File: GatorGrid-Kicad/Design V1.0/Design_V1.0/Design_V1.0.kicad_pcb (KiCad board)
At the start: 2 copper layers, 95 x 63 mm, 10 parts, among them J1 Conn_01x02, U1 TP4056

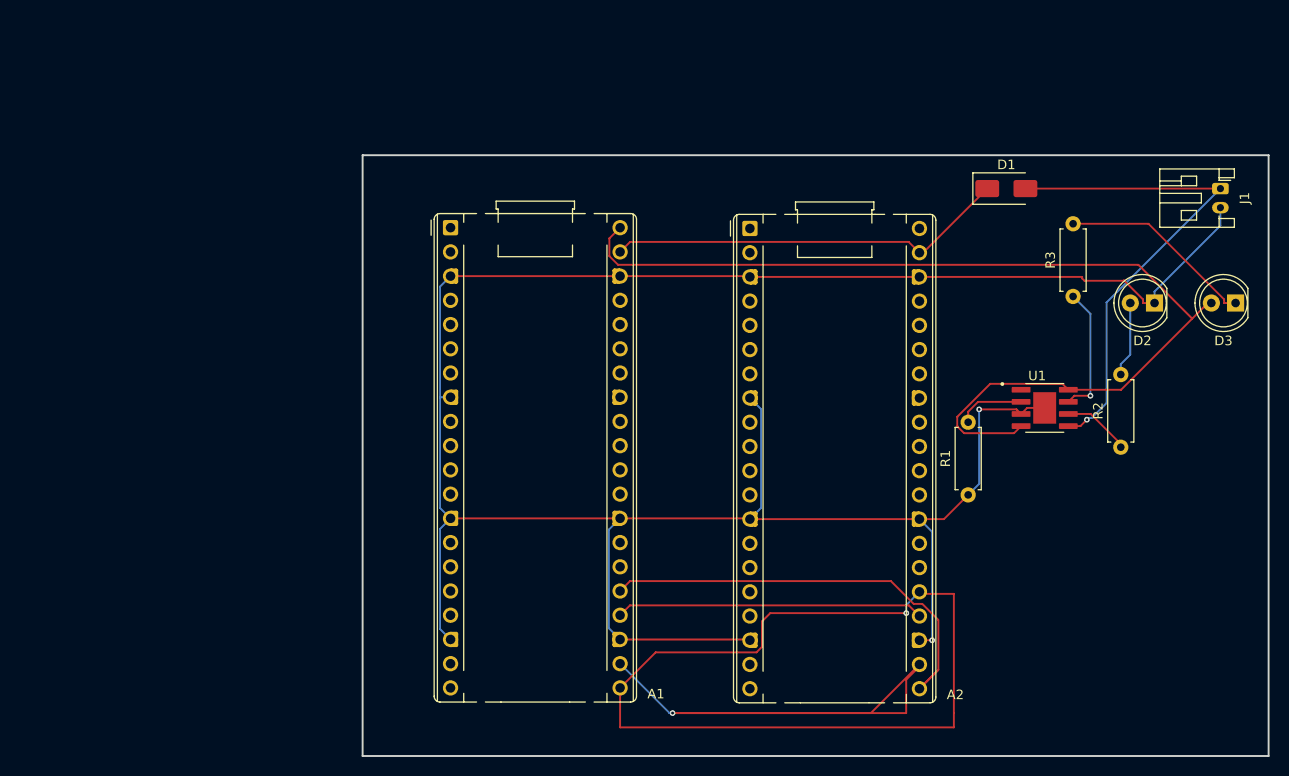
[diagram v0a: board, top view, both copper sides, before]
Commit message: updated PCB
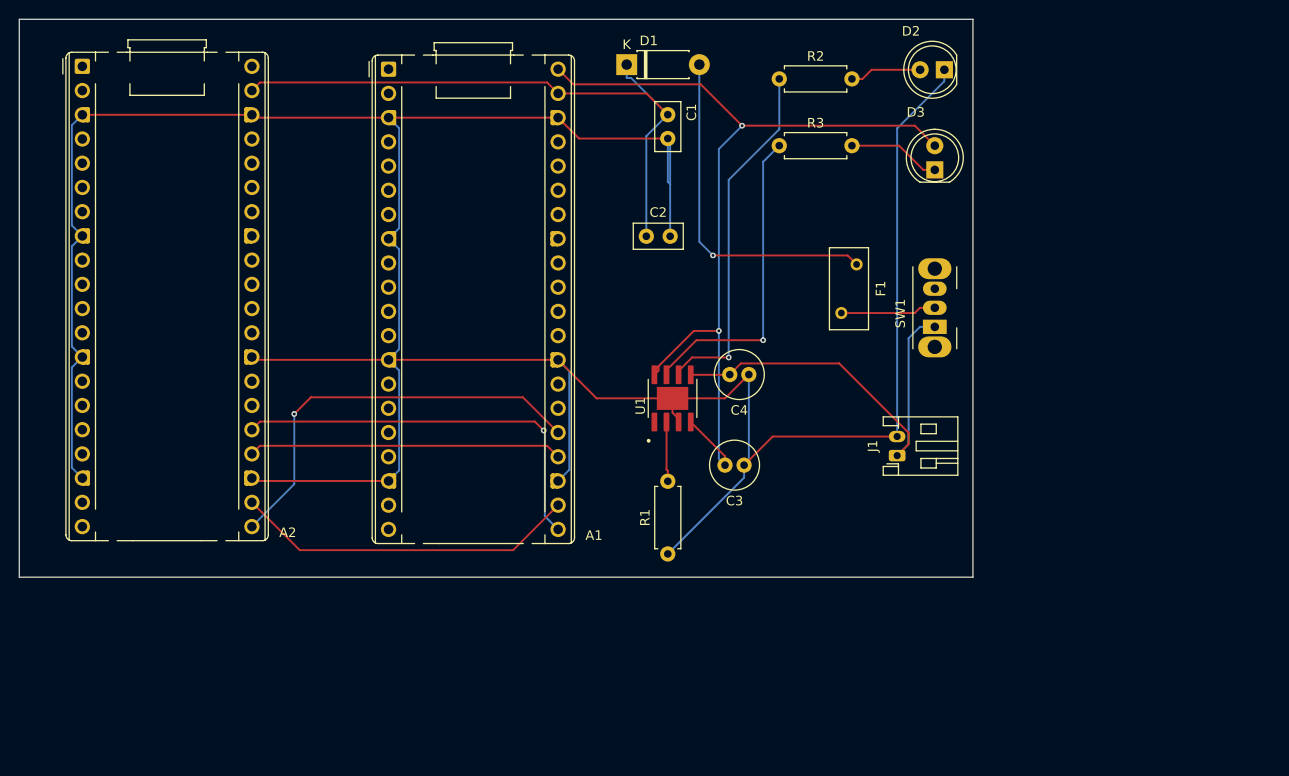
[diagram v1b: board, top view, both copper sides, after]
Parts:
- added C1: 100nF, Capacitor_THT:C_Disc_D5.0mm_W2.5mm_P2.50mm, F.Cu at (106.5, 40.8)
- added C2: 100nF, Capacitor_THT:C_Disc_D5.0mm_W2.5mm_P2.50mm, F.Cu at (104.2, 53.5)
- added C3: 10uF, Capacitor_THT:C_Radial_D5.0mm_H11.0mm_P2.00mm, F.Cu at (114.5, 77.5)
- added C4: 10uF, Capacitor_THT:C_Radial_D5.0mm_H11.0mm_P2.00mm, F.Cu at (115.0, 68.0)
- added F1: Polyfuse, Fuse:Fuse_BelFuse_0ZRE0005FF_L8.3mm_W3.8mm, F.Cu at (126.3, 56.5)
- added SW1: SW_SPST, Button_Switch_THT:SW_Slide_SPDT_Angled_CK_OS102011MA1Q, F.Cu at (134.5, 63.0)
- A1: value RaspberryPi_Pico -> RPICO-AP
- A2: value RaspberryPi_Pico -> RPICO-STA
- D1: footprint Diode_SMD:D_SMA -> Diode_THT:D_DO-41_SOD81_P7.62mm_Horizontal
- J1: value Conn_01x02 -> Battery-Connector
- moved A2 72.0 mm to (45.1, 35.7)
- moved R2 52.7 mm to (118.2, 37.0), turned to 0 degrees
- moved J1 44.0 mm to (130.6, 76.5), turned to 90 degrees
- moved D1 41.9 mm to (102.2, 35.5)
- moved U1 39.0 mm to (107.0, 70.5), turned to 90 degrees
- moved R3 34.6 mm to (118.2, 44.0), turned to 0 degrees
- moved D3 34.5 mm to (134.5, 46.5), turned to 90 degrees
- moved D2 32.9 mm to (135.5, 36.0)
- moved R1 32.1 mm to (106.5, 86.8)
- moved A1 17.8 mm to (77.2, 36.0)
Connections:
- D1 pad 2: VBAT(+) -> Net-(D1-A)
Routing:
- net GND: track 257.6 -> 324.9 mm, vias 2 -> 0
- net Net-(D1-A): track 0.00 -> 36.1 mm, vias 0 -> 1
- net STDBY: track 7.14 -> 37.6 mm, vias 0 -> 1
- net VSYS: track 42.2 -> 66.3 mm
- net CHRG: track 13.8 -> 33.0 mm
- net VBUS: track 107.8 -> 95.3 mm, vias 0 -> 2
- net Net-(D3-K): track 20.7 -> 9.74 mm
- net Net-(SW1-B): track 0.00 -> 10.0 mm
- net VBAT(+): track 52.8 -> 45.3 mm, vias 1 -> 0
- net RX-TX: track 37.6 -> 42.3 mm
- net TX-RX: track 46.2 -> 43.6 mm, vias 0 -> 1
- net Net-(U1-PROG): track 7.08 -> 6.27 mm
- net SCK: track 32.3 -> 32.9 mm
- net CS: track 35.6 -> 36.1 mm, vias 1 -> 0
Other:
- board size 95 x 63 mm -> 100 x 58.5 mm
